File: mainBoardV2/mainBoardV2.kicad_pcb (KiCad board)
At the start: 2 copper layers, 55.9 x 117 mm, 28 parts, among them J1 USB4125-GF-A_REVA2, U2 ESP32-DEVKITC-32E, U3 MCP73871-2AAI_ML, U4 MPU6050_Module, U5 TPS61023DRLT

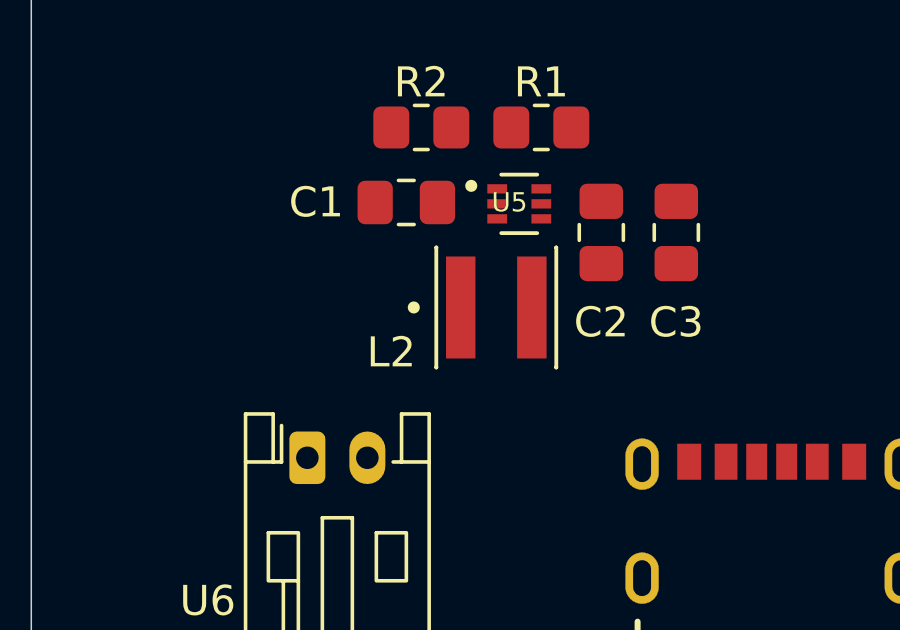
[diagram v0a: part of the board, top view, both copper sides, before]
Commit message: 3.11.26.C1
False Start
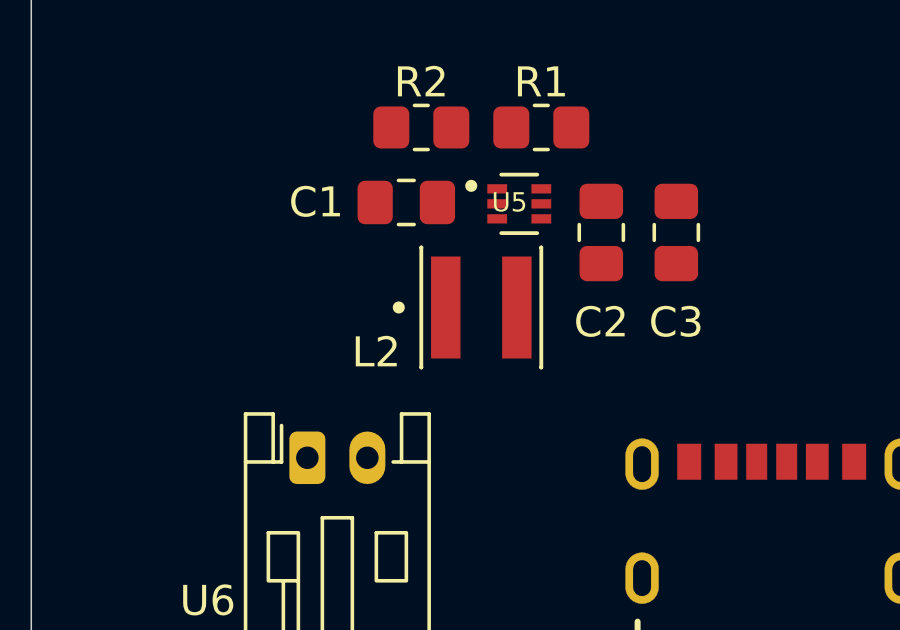
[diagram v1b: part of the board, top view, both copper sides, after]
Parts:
- moved L2 0.50 mm to (97.0, 117.0)
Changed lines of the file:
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@@
 	(footprint "XEL4030-102MEC:IND_XEL4030-102MEC"
 		(layer "F.Cu")
-		(at 97.5 117)
+		(at 97 117)
 		(property "Reference" "L2"
 			(at -3.5 1.5 0)
